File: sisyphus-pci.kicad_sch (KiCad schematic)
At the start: 124 parts, among them J1 Bus_PCI_32bit_Universal, J10 LINE_OUT, J2 JOYSTICK, J3 CD_IN, J4 WAVE_BLASTER, J5 LINE_IN_HDR, J6 LINE_IN_3.5, J7 HEADPHONE_OUT, J8 PCPCI, J9 LINE_OUT_3.5M, Q1 BF545A, U1 ES1938_PCI, U2 BA4564, U3 LF50_TO252, U4 LM4880, U6 L79L05_SOIC-8, Y1 14.318MHz

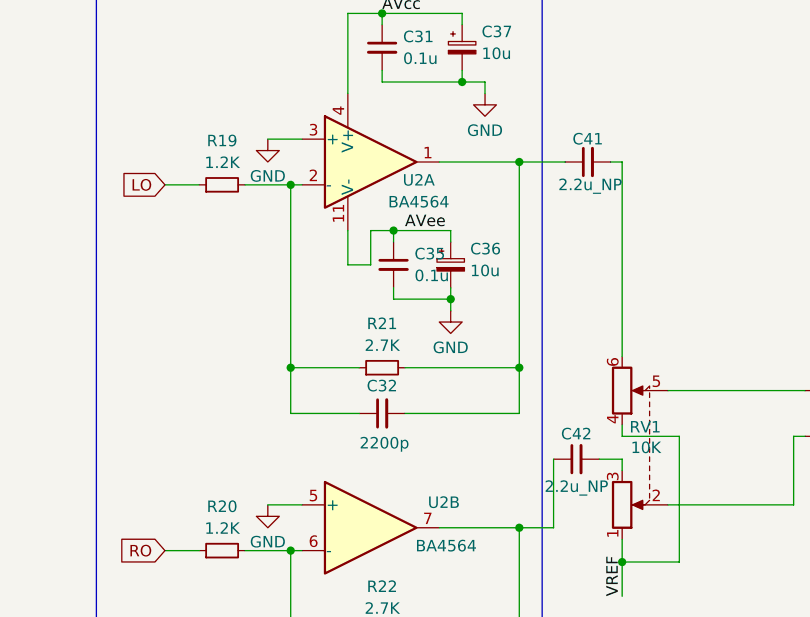
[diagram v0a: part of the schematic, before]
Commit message: Add files via upload
Updated to version 0.1a
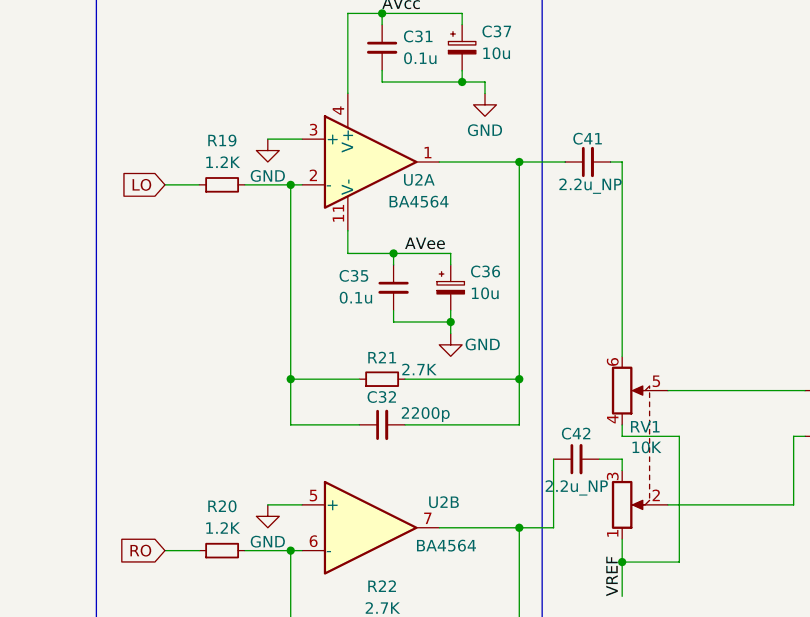
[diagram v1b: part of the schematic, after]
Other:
- moved on the sheet: C32, C35, C36, R21
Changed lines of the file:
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@@
 	)
 	(junction
-		(at 396.24 57.15)
+		(at 396.24 58.42)
 		(diameter 0)
 		(color 0 0 0 0)
@@
 	)
 	(junction
-		(at 388.62 49.53)
+		(at 388.62 52.07)
 		(diameter 0)
 		(color 0 0 0 0)
@@
 	)
 	(junction
-		(at 382.27 41.91)
+		(at 382.27 44.45)
 		(diameter 0)
 		(color 0 0 0 0)
@@
 	)
 	(junction
-		(at 370.84 57.15)
+		(at 370.84 58.42)
 		(diameter 0)
 		(color 0 0 0 0)
@@
 	(wire
 		(pts
-			(xy 382.27 48.26) (xy 382.27 49.53)
+			(xy 382.27 50.8) (xy 382.27 52.07)
 		)
 		(stroke
@@
 	(wire
 		(pts
-			(xy 396.24 34.29) (xy 396.24 57.15)
+			(xy 396.24 34.29) (xy 396.24 58.42)
 		)
 		(stroke
@@
 	(wire
 		(pts
-			(xy 377.19 45.72) (xy 379.73 45.72)
+			(xy 377.19 44.45) (xy 382.27 44.45)
 		)
 		(stroke
@@
 	(wire
 		(pts
-			(xy 370.84 62.23) (xy 378.46 62.23)
+			(xy 370.84 63.5) (xy 378.46 63.5)
 		)
 		(stroke
@@
 	(wire
 		(pts
-			(xy 388.62 41.91) (xy 388.62 43.18)
+			(xy 388.62 44.45) (xy 388.62 45.72)
 		)
 		(stroke
@@
 	(wire
 		(pts
-			(xy 382.27 41.91) (xy 388.62 41.91)
+			(xy 382.27 44.45) (xy 388.62 44.45)
 		)
 		(stroke
@@
 	(wire
 		(pts
-			(xy 379.73 45.72) (xy 379.73 41.91)
-		)
-		(stroke
-			(width 0)
-			(type default)
-		)
-	)
-	(wire
-		(pts
 			(xy 90.17 34.29) (xy 101.6 34.29)
 		)
@@
 	(wire
 		(pts
-			(xy 377.19 41.91) (xy 377.19 45.72)
+			(xy 377.19 41.91) (xy 377.19 44.45)
 		)
 		(stroke
@@
 	(wire
 		(pts
-			(xy 379.73 41.91) (xy 382.27 41.91)
-		)
-		(stroke
-			(width 0)
-			(type default)
-		)
-	)
-	(wire
-		(pts
 			(xy 252.73 163.83) (xy 259.08 163.83)
 		)
@@
 	(wire
 		(pts
-			(xy 370.84 57.15) (xy 378.46 57.15)
+			(xy 370.84 58.42) (xy 378.46 58.42)
 		)
 		(stroke
@@
 	(wire
 		(pts
-			(xy 388.62 49.53) (xy 388.62 50.8)
+			(xy 388.62 52.07) (xy 388.62 53.34)
 		)
 		(stroke
@@
 	(wire
 		(pts
-			(xy 382.27 49.53) (xy 388.62 49.53)
+			(xy 382.27 52.07) (xy 388.62 52.07)
 		)
 		(stroke
@@
 	(wire
 		(pts
-			(xy 382.27 41.91) (xy 382.27 43.18)
+			(xy 382.27 44.45) (xy 382.27 45.72)
 		)
 		(stroke
@@
 	(wire
 		(pts
-			(xy 396.24 62.23) (xy 396.24 57.15)
+			(xy 396.24 63.5) (xy 396.24 58.42)
 		)
 		(stroke
@@
 	(wire
 		(pts
-			(xy 383.54 62.23) (xy 396.24 62.23)
+			(xy 383.54 63.5) (xy 396.24 63.5)
 		)
 		(stroke
@@
 	(wire
 		(pts
-			(xy 396.24 57.15) (xy 383.54 57.15)
+			(xy 396.24 58.42) (xy 383.54 58.42)
 		)
 		(stroke
@@
 	(wire
 		(pts
-			(xy 370.84 57.15) (xy 370.84 62.23)
+			(xy 370.84 58.42) (xy 370.84 63.5)
 		)
 		(stroke
@@
 	(wire
 		(pts
-			(xy 370.84 36.83) (xy 370.84 57.15)
+			(xy 370.84 36.83) (xy 370.84 58.42)
 		)
 		(stroke
@@
 	(wire
 		(pts
-			(xy 388.62 48.26) (xy 388.62 49.53)
+			(xy 388.62 50.8) (xy 388.62 52.07)
 		)
 		(stroke
@@
 	)
 	(label "AVee"
-		(at 383.54 41.91 0)
+		(at 383.54 44.45 0)
 		(fields_autoplaced yes)
 		(effects
@@
 	(symbol
 		(lib_id "Device:C_Small")
-		(at 382.27 45.72 0)
+		(at 382.27 48.26 0)
 		(unit 1)
 		(exclude_from_sim no)
@@
 		(on_board yes)
 		(dnp no)
-		(fields_autoplaced yes)
 		(property "Reference" "C35"
-			(at 384.5941 44.5141 0)
+			(at 376.174 46.99 0)
 			(effects
 				(font
@@
 		)
 		(property "Value" "0.1u"
-			(at 384.5941 46.9384 0)
+			(at 376.174 49.4143 0)
 			(effects
 				(font
@@
 		)
 		(property "Footprint" "Capacitor_SMD:C_0805_2012Metric"
-			(at 382.27 45.72 0)
+			(at 382.27 48.26 0)
 			(effects
 				(font
@@
 		)
 		(property "Datasheet" "~"
-			(at 382.27 45.72 0)
+			(at 382.27 48.26 0)
 			(effects
 				(font
@@
 		)
 		(property "Description" "Unpolarized capacitor, small symbol"
-			(at 382.27 45.72 0)
+			(at 382.27 48.26 0)
 			(effects
 				(font
@@
 	(symbol
 		(lib_id "Device:C_Polarized_Small")
-		(at 388.62 45.72 0)
+		(at 388.62 48.26 0)
 		(unit 1)
 		(exclude_from_sim no)
@@
 		(fields_autoplaced yes)
 		(property "Reference" "C36"
-			(at 390.779 43.9617 0)
+			(at 390.779 46.5017 0)
 			(effects
 				(font
@@
 		)
 		(property "Value" "10u"
-			(at 390.779 46.386 0)
+			(at 390.779 48.926 0)
 			(effects
 				(font
@@
 		)
 		(property "Footprint" "Capacitor_SMD:C_1206_3216Metric"
-			(at 388.62 45.72 0)
+			(at 388.62 48.26 0)
 			(effects
 				(font
@@
 		)
 		(property "Datasheet" "~"
-			(at 388.62 45.72 0)
+			(at 388.62 48.26 0)
 			(effects
 				(font
@@
 		)
 		(property "Description" "Polarized capacitor, small symbol"
-			(at 388.62 45.72 0)
+			(at 388.62 48.26 0)
 			(effects
 				(font
@@
 	(symbol
 		(lib_id "Device:R_Small")
-		(at 381 57.15 90)
+		(at 381 58.42 90)
 		(unit 1)
 		(exclude_from_sim no)
@@
 		(on_board yes)
 		(dnp no)
-		(fields_autoplaced yes)
 		(property "Reference" "R21"
-			(at 381 52.2689 90)
+			(at 381 56.0789 90)
 			(effects
 				(font
@@
 		)
 		(property "Value" "2.7K"
-			(at 381 54.6932 90)
+			(at 385.064 57.404 90)
 			(effects
 				(font
@@
 		)
 		(property "Footprint" "Resistor_SMD:R_0805_2012Metric"
-			(at 381 57.15 0)
+			(at 381 58.42 0)
 			(effects
 				(font
@@
 		)
 		(property "Datasheet" "~"
-			(at 381 57.15 0)
+			(at 381 58.42 0)
 			(effects
 				(font
@@
 		)
 		(property "Description" "Resistor, small symbol"
-			(at 381 57.15 0)
+			(at 381 58.42 0)
 			(effects
 				(font
@@
 	(symbol
 		(lib_id "power:GND")
-		(at 388.62 50.8 0)
+		(at 388.62 53.34 0)
 		(unit 1)
 		(exclude_from_sim no)
@@
 		(on_board yes)
 		(dnp no)
-		(fields_autoplaced yes)
 		(property "Reference" "#PWR016"
-			(at 388.62 57.15 0)
+			(at 388.62 59.69 0)
 			(effects
 				(font
@@
 		)
 		(property "Value" "GND"
-			(at 388.62 54.9331 0)
+			(at 392.176 54.61 0)
 			(effects
 				(font
@@
 		)
 		(property "Footprint" ""
-			(at 388.62 50.8 0)
+			(at 388.62 53.34 0)
 			(effects
 				(font
@@
 		)
 		(property "Datasheet" ""
-			(at 388.62 50.8 0)
+			(at 388.62 53.34 0)
 			(effects
 				(font
@@
 		)
 		(property "Description" "Power symbol creates a global label with name \"GND\" , ground"
-			(at 388.62 50.8 0)
+			(at 388.62 53.34 0)
 			(effects
 				(font
@@
 	(symbol
 		(lib_id "Device:C_Small")
-		(at 381 62.23 90)
+		(at 381 63.5 90)
 		(unit 1)
 		(exclude_from_sim no)
@@
 		(dnp no)
 		(property "Reference" "C32"
-			(at 381 59.182 90)
+			(at 381 60.452 90)
 			(effects
 				(font
@@
 		)
 		(property "Value" "2200p"
-			(at 381.254 65.532 90)
+			(at 385.826 62.23 90)
 			(effects
 				(font
@@
 		)
 		(property "Footprint" "Capacitor_SMD:C_0805_2012Metric"
-			(at 381 62.23 0)
+			(at 381 63.5 0)
 			(effects
 				(font
@@
 		)
 		(property "Datasheet" "~"
-			(at 381 62.23 0)
+			(at 381 63.5 0)
 			(effects
 				(font
@@
 		)
 		(property "Description" "Unpolarized capacitor, small symbol"
-			(at 381 62.23 0)
+			(at 381 63.5 0)
 			(effects
 				(font
